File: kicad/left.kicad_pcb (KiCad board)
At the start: 4 copper layers, 127.3 x 89.6 mm, 159 parts, among them M2 MountingHole_2.2mm_M2, Q1 PMF170XP,115, Q2 FS8205A_C2830320, SW1 TS-1088-AR02016, U1 TLV7031QDCKRQ1, U2 E73-2G4M08S1C, U3 SN74LVC1G74DQER, U4 BL8573CS8TR, U4 S2B-PH-K-S(LF)(SN), U7 LP5024RSMR, U8 DW01A_C42380662, X1 FC-13532.768KHZ9PF20PPM

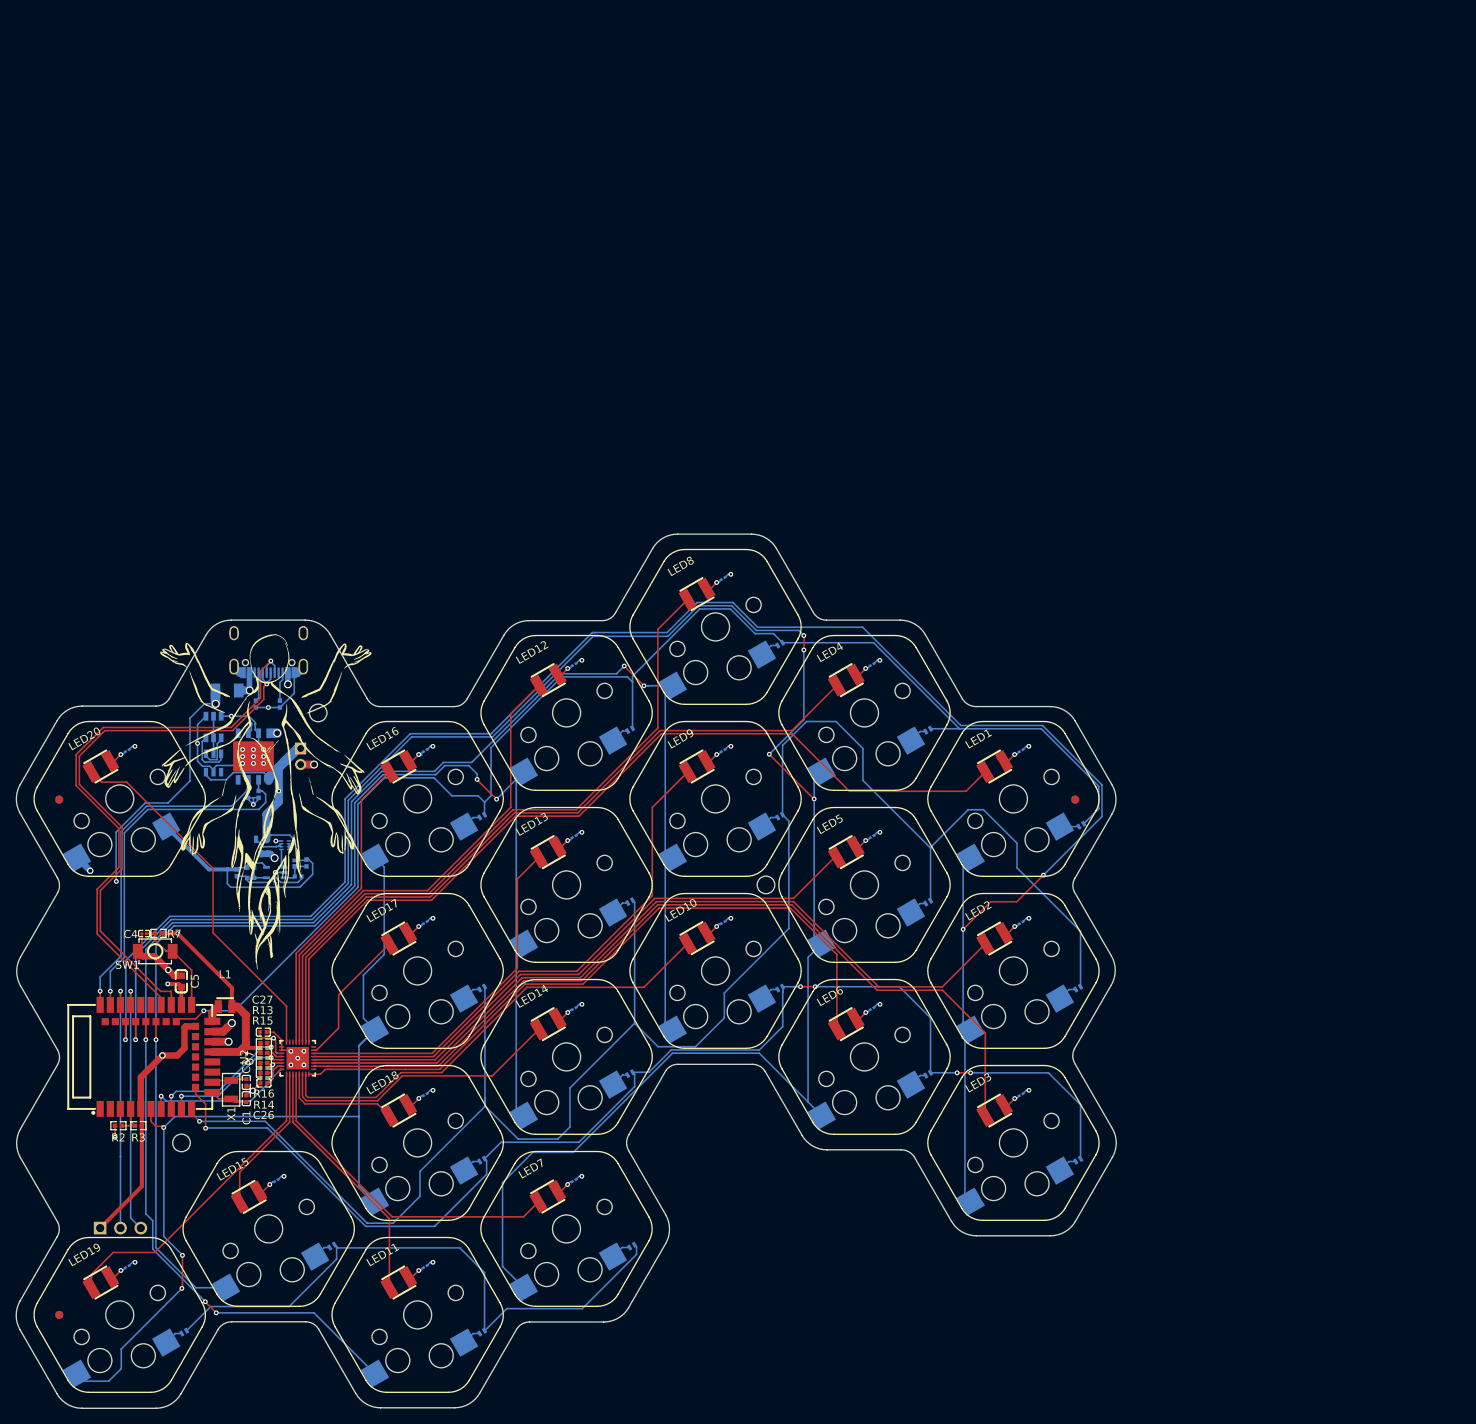
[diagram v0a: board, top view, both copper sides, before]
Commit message: finished right, i hope
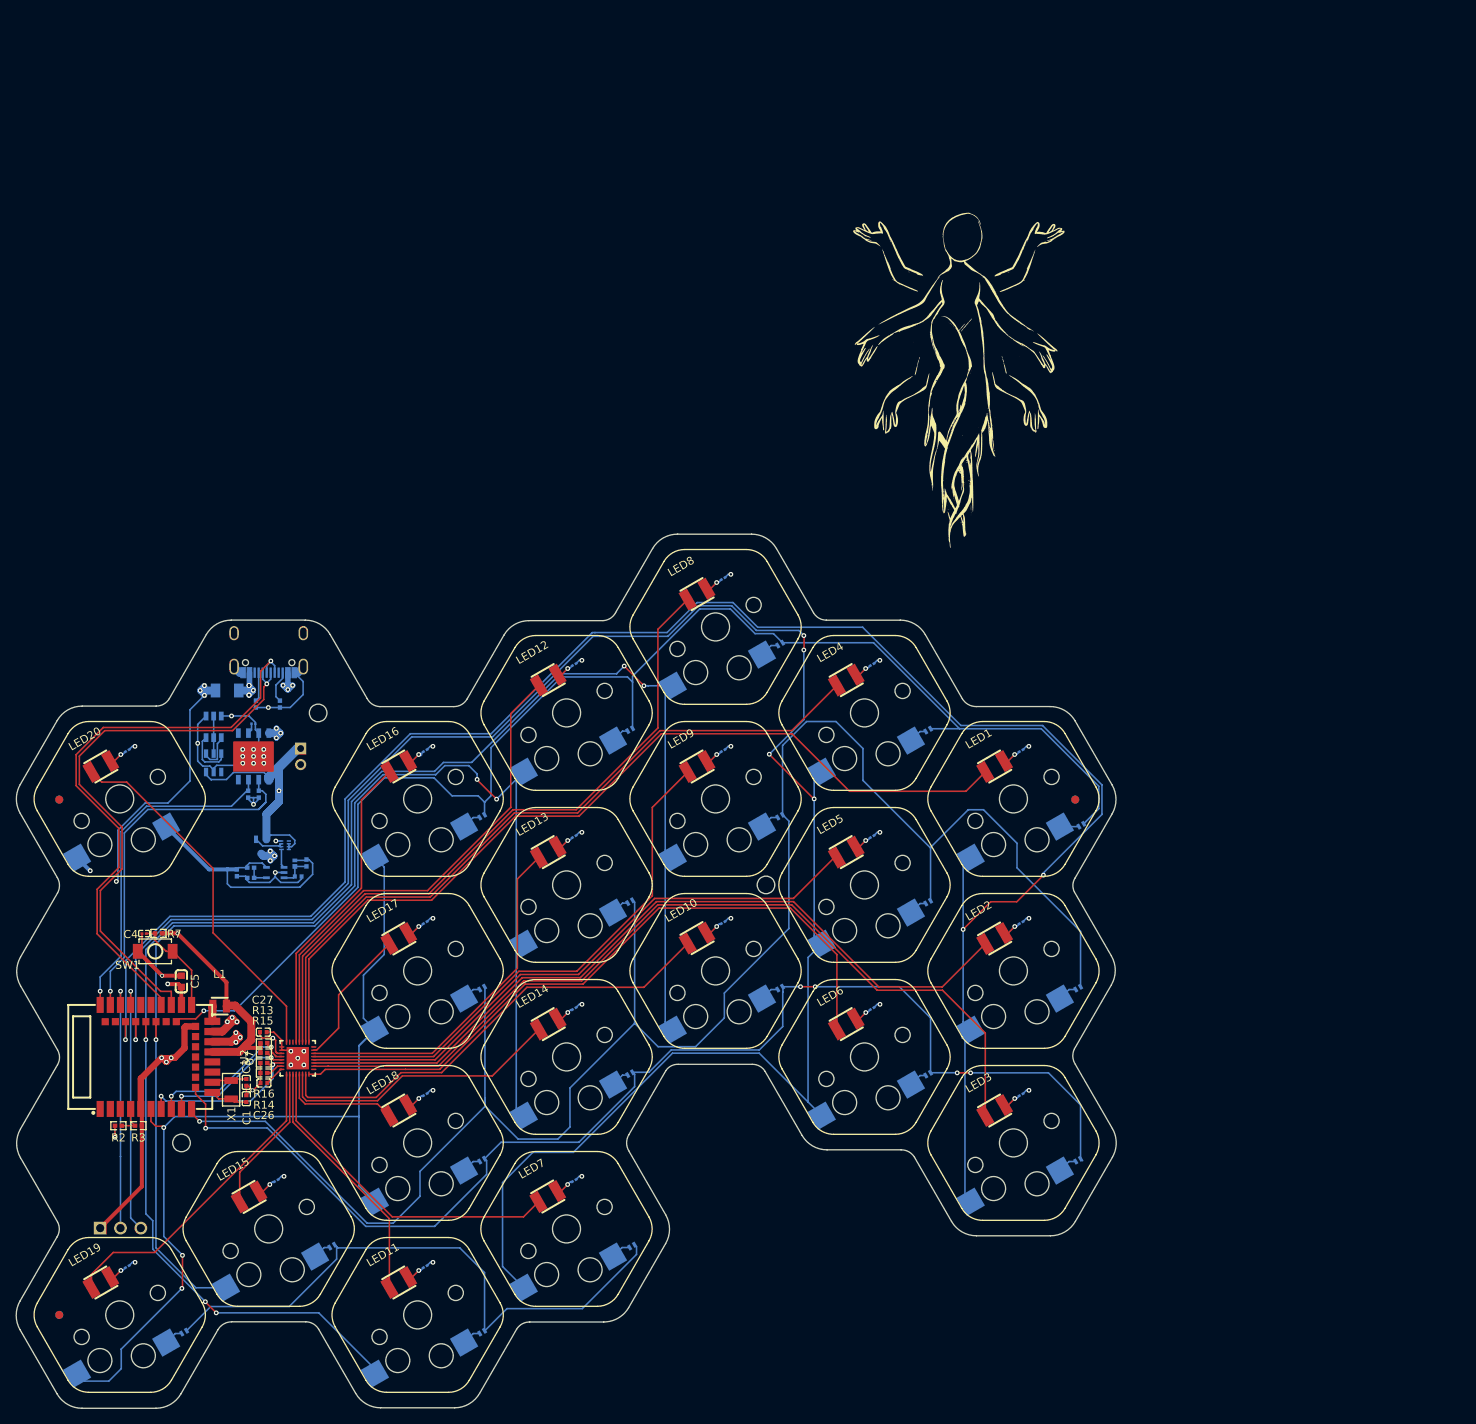
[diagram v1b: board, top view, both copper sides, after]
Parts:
- removed the U4 at (49.7, 43.6)
- removed U8: DW01A_C42380662, easyeda2kicad:SOT-23-6_L2.9-W1.6-P0.95-LS2.9-BL
- added U5: BL8573CS8TR, easyeda2kicad:ESOP-8_L4.9-W3.9-P1.27-LS6.0-BL-EP, B.Cu at (49.7, 43.6)
- added U6: DW01A_C42380662, easyeda2kicad:SOT-23-6_L2.9-W1.6-P0.95-LS2.9-BL, B.Cu at (44.7, 44.4)
- moved G*** 166.0 mm to (252.3, -6.80)
- moved G*** 166.0 mm to (262.7, 81.2)
- moved G** 101.4 mm to (142.5, -16.2)
- moved L1 0.68 mm to (45.5, 74.8)
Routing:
- net /VBUS: track 61.9 -> 74.8 mm, vias 4 -> 8
- net Net-(F1-Pad1): track 10.7 -> 21.0 mm, vias 2 -> 8
- net GND: track 119.3 -> 125.0 mm, vias 44 -> 47
- net /PWR: track 87.3 -> 92.5 mm, vias 24 -> 28
- net /STDBY: track 44.9 -> 46.2 mm
- net /BAT+: track 61.7 -> 62.8 mm
- net /VDD_nRF: track 53.1 -> 54.0 mm

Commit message: started left
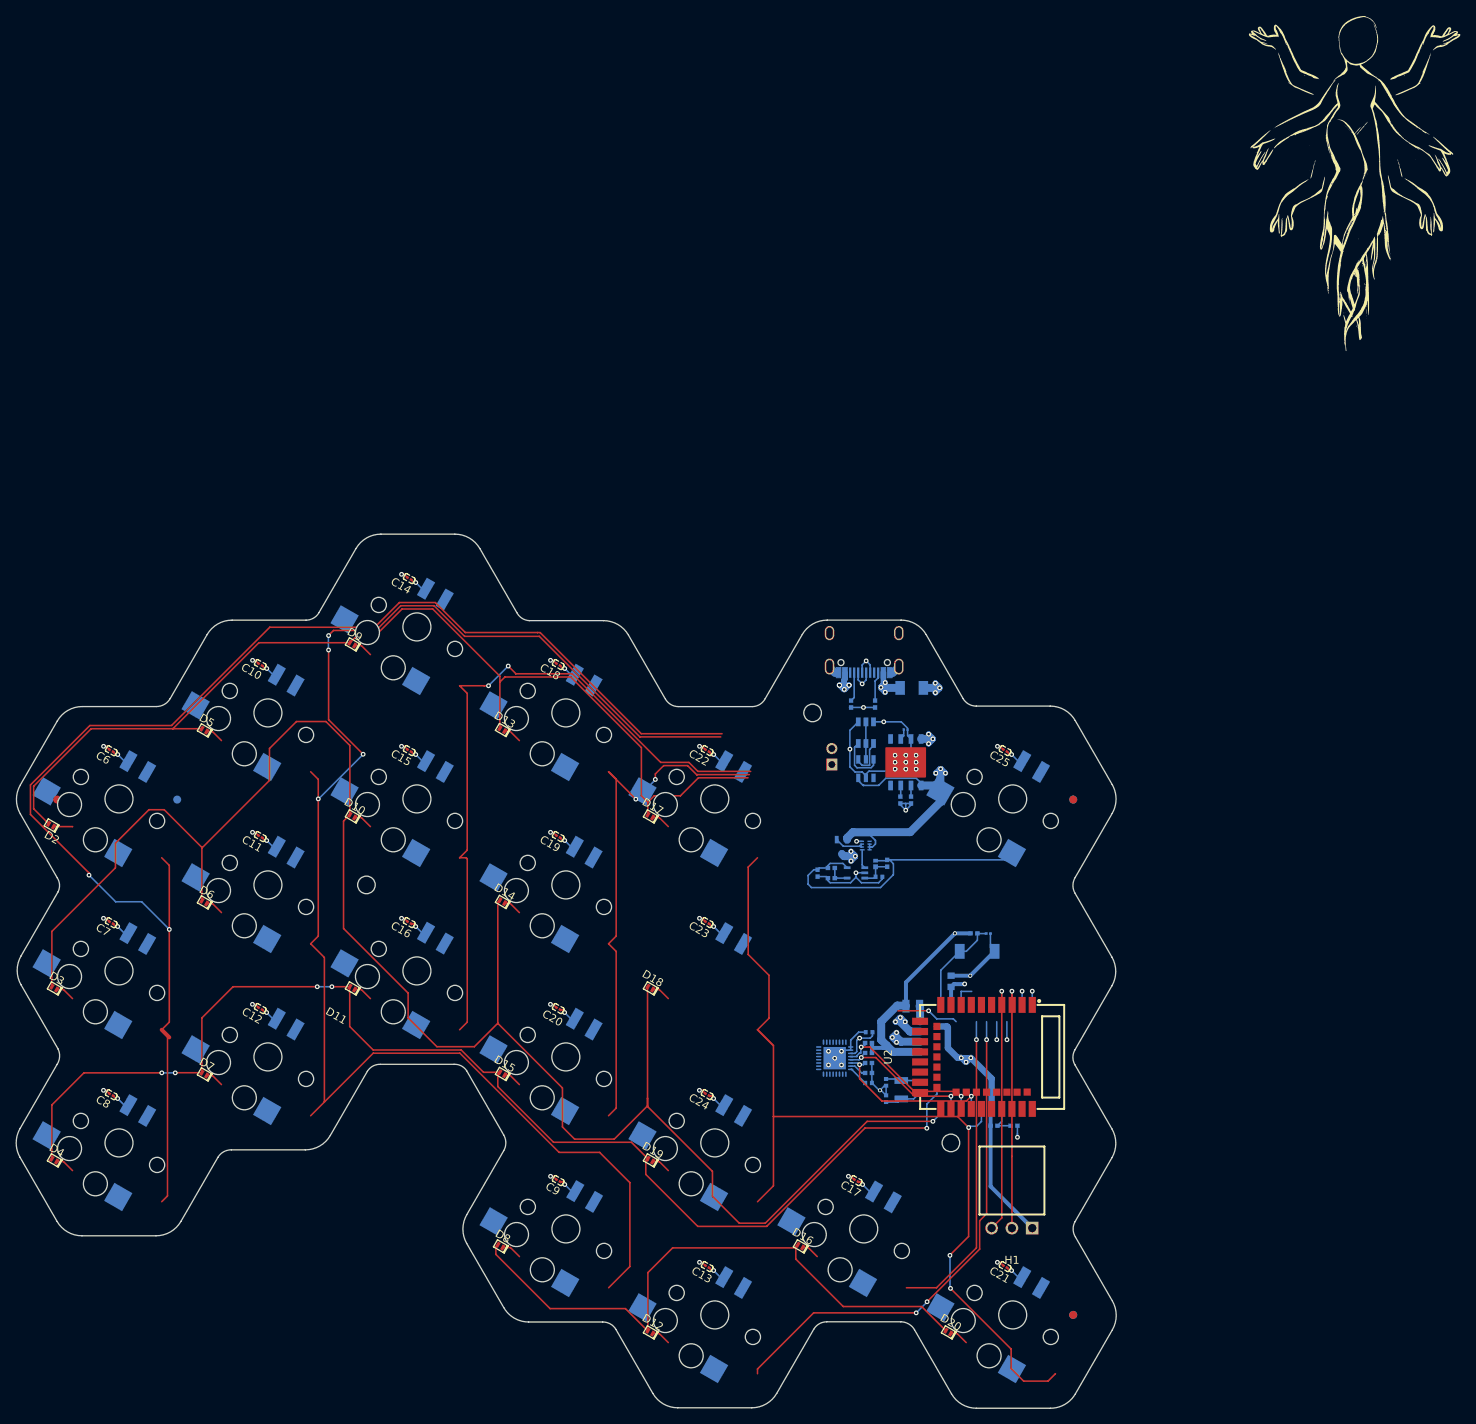
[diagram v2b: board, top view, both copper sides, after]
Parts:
- removed S17: Choc HEX, hexcaps:PG1350_hotswap
- C1, C26, C27, C3, C4, C5, Fi4, Fi5, Fi6, L1, LED1, LED10, LED11, LED12, LED13, LED14, LED15, LED16, LED17, LED18, LED19, LED2, LED20, LED3, LED4, LED5, LED6, LED7, LED8, LED9, M2, R13, R14, R15, R16, R2, R3, R7, REF** (x2), SW1, U7, X1, hex_edge (x18): moved to B.Cu
- C10, C11, C12, C13, C14, C15, C16, C17, C18, C19, C20, C21, C22, C23, C24, C25, C6, C7, C8, C9, D10, D11, D12, D13, D14, D15, D16, D17, D18, D19, D2, D20, D3, D4, D5, D6, D7, D8, D9, Fi1, Fi2, Fi3, H1: moved to F.Cu
- S1, S10, S11, S12, S13, S14, S15, S16, S18, S19, S2, S20, S3, S4, S5, S6, S7, S8, S9: footprint hexcaps:PG1350_hotswap -> hexcaps:PG1350_hotswap_reversed; moved to F.Cu
- moved D2 128.8 mm to (24.4, 52.2), turned to 150 degrees
- moved D3 128.0 mm to (24.8, 72.6), turned to 150 degrees
- moved D4 128.0 mm to (24.8, 94.1), turned to 150 degrees
- moved Fi2 127.3 mm to (25.2, 49.0), turned to 0 degrees
- moved Fi1 126.7 mm to (152.2, 49.0), turned to 0 degrees
- moved Fi3 126.7 mm to (152.2, 113.4), turned to 0 degrees
- moved Fi4 126.7 mm to (152.2, 49.0), turned to 180 degrees
- moved Fi6 126.7 mm to (152.2, 113.4), turned to 180 degrees
- moved LED19 116.4 mm to (147.0, 109.4), turned to 150 degrees
- moved LED20 116.4 mm to (147.0, 44.9), turned to 150 degrees
- moved C6 113.7 mm to (31.9, 42.9), turned to 150 degrees
- moved C7 113.7 mm to (31.9, 64.4), turned to 150 degrees
- moved C8 113.7 mm to (31.9, 85.9), turned to 150 degrees
- moved Fi5 112.3 mm to (40.2, 49.0), turned to 180 degrees
- moved R2 111.9 mm to (144.8, 89.8), turned to 0 degrees
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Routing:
- net /COL2: track 253.5 -> 0.00 mm, vias 5 -> 0
- net /COL1: track 241.2 -> 0.00 mm, vias 3 -> 0
- net /ROW3: track 156.1 -> 334.0 mm, vias 5 -> 8
- net /COL3: track 207.4 -> 342.4 mm, vias 5 -> 10
- net /COL4: track 160.6 -> 39.1 mm, vias 3 -> 1
- net /LED1: track 110.6 -> 0.00 mm
- net /LED3: track 109.3 -> 0.00 mm
- net /LED2: track 98.9 -> 0.00 mm
- net /LED4: track 91.1 -> 0.00 mm
- net /LED6: track 86.4 -> 0.00 mm
- net /LED8: track 84.6 -> 0.00 mm
- net /CHRG: track 42.1 -> 122.2 mm, vias 1 -> 4
- net /LED5: track 75.9 -> 0.00 mm
- net /D+: track 72.2 -> 3.34 mm
- net /LED9: track 68.0 -> 0.00 mm
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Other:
- outline, holes or cut-outs redrawn
